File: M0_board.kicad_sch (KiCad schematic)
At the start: 88 parts, among them J301 Screw_Terminal_01x01, J302 Screw_Terminal_01x01, J303 Conn_01x05_MountingPin, J304 X4621WVS-2x20I-C40D64, J305 X4621FVS-2x20-C43D65, J306 Screw_Terminal_01x01, J307 Screw_Terminal_01x01, J309 Screw_Terminal_01x01, Q301 HYG025N06LS1C2, Q302 HYG025N06LS1C2, Q303 HYG025N06LS1C2, Q304 HYG025N06LS1C2, Q305 HYG025N06LS1C2, Q306 HYG025N06LS1C2, Q307 HYG025N06LS1C2, Q308 HYG025N06LS1C2, Q309 HYG025N06LS1C2, Q310 HYG025N06LS1C2, Q311 HYG025N06LS1C2, Q312 HYG025N06LS1C2, U301 DRV8301DCAR

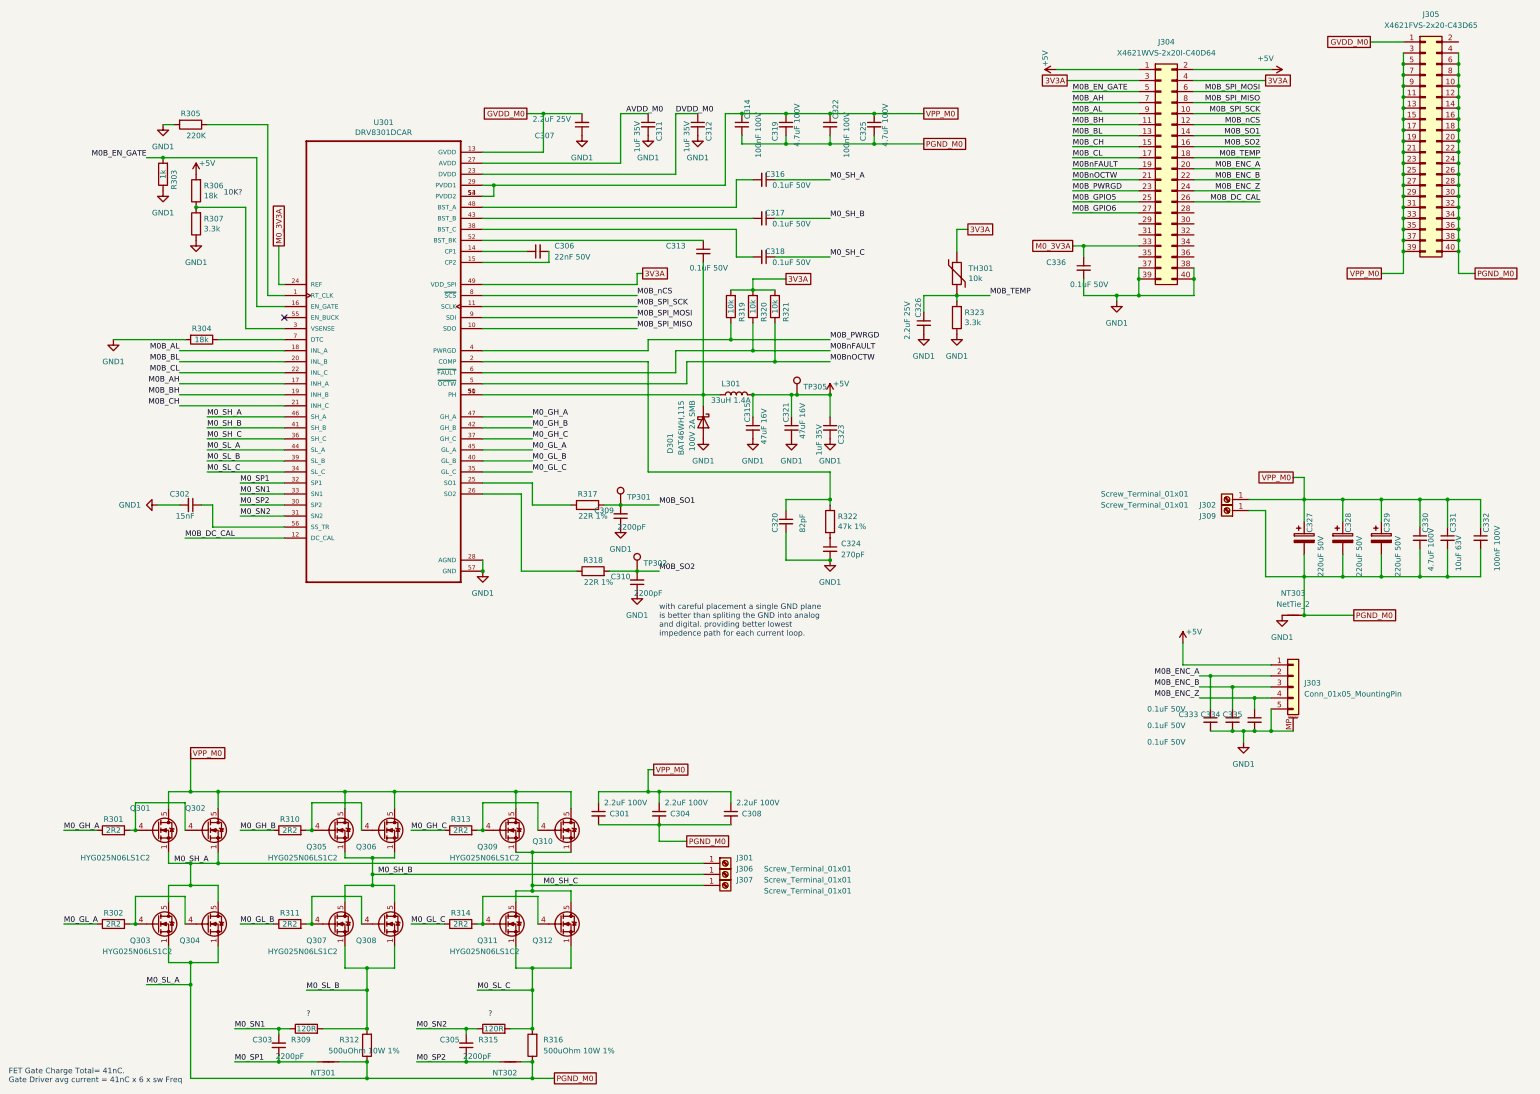
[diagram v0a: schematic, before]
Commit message: Update artwork for M0 board
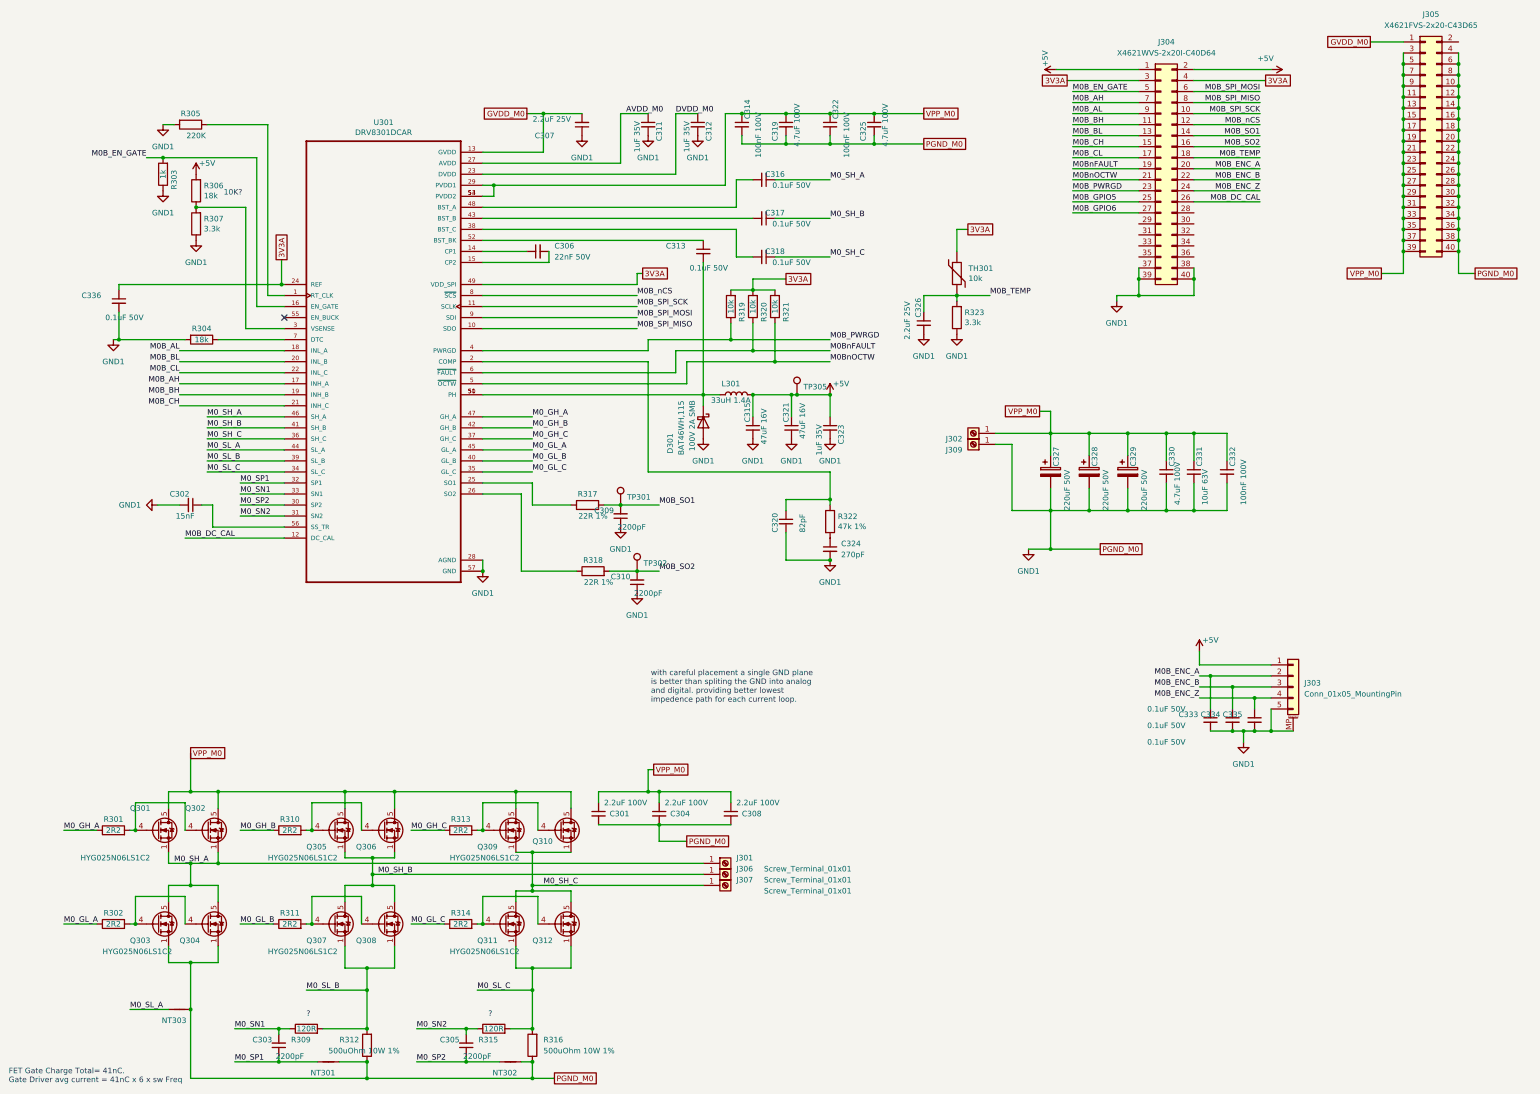
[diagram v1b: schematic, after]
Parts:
- removed NT303: NetTie_2, qdrive_footprints:NetTie-2_SMD_Pad2.0mm, symbol Device:NetTie_2
- added NT303: Net-Tie_2, NetTie:NetTie-2_SMD_Pad0.5mm, symbol bldc_motor_cntroller-rescue:Net-Tie_2-Device
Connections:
- net 3V3A: now also C336.1, U301.24 (REF)
- net GND1: now also C301.2, C304.2, C308.2, C314.2, C319.2, C322.2, C325.2, C327.2, C328.2, C329.2, C330.2, C331.2, C332.2, J305.10 (Pin_10), J305.12 (Pin_12), J305.14 (Pin_14), J305.16 (Pin_16), J305.18 (Pin_18), J305.20 (Pin_20), J305.22 (Pin_22), J305.24 (Pin_24), J305.26 (Pin_26), J305.28 (Pin_28), J305.30 (Pin_30), J305.32 (Pin_32), J305.34 (Pin_34), J305.36 (Pin_36), J305.38 (Pin_38), J305.4 (Pin_4), J305.40 (Pin_40), J305.6 (Pin_6), J305.8 (Pin_8), J309.1 (Pin_1), NT301.2, NT302.2, Q303.1 (S), Q303.2 (S), Q303.3 (S), Q304.1 (S), Q304.2 (S), Q304.3 (S), R312.1, R316.1, NT303.2
- removed net M0_3V3A: C336.1, J304.33 (Pin_33), U301.24 (REF)
- removed net PGND_M0: C301.2, C304.2, C308.2, C314.2, C319.2, C322.2, C325.2, C327.2, C328.2, C329.2, C330.2, C331.2, C332.2, J305.10 (Pin_10), J305.12 (Pin_12), J305.14 (Pin_14), J305.16 (Pin_16), J305.18 (Pin_18), J305.20 (Pin_20), J305.22 (Pin_22), J305.24 (Pin_24), J305.26 (Pin_26), J305.28 (Pin_28), J305.30 (Pin_30), J305.32 (Pin_32), J305.34 (Pin_34), J305.36 (Pin_36), J305.38 (Pin_38), J305.4 (Pin_4), J305.40 (Pin_40), J305.6 (Pin_6), J305.8 (Pin_8), J309.1 (Pin_1), NT301.2, NT302.2, Q303.1 (S), Q303.2 (S), Q303.3 (S), Q304.1 (S), Q304.2 (S), Q304.3 (S), R312.1, R316.1, U301.44 (SL_A)
- new net M0_SL_A: NT303.1, U301.44 (SL_A)
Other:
- moved on the sheet: C327, C328, C329, C330, C331, C332, C336, J302, J309
